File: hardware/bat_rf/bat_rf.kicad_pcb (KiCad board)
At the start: 2 copper layers, 89.8 x 41.5 mm, 95 parts, among them J1 USB_C_Receptacle_PowerOnly_6P, J2 Conn_01x04, J4 Conn_01x02, Q1 NMOS, SW2 RESET, U1 TPS54331, U2 IP2325_5M_WHJC, U3 ESP8684-WROOM-02UC

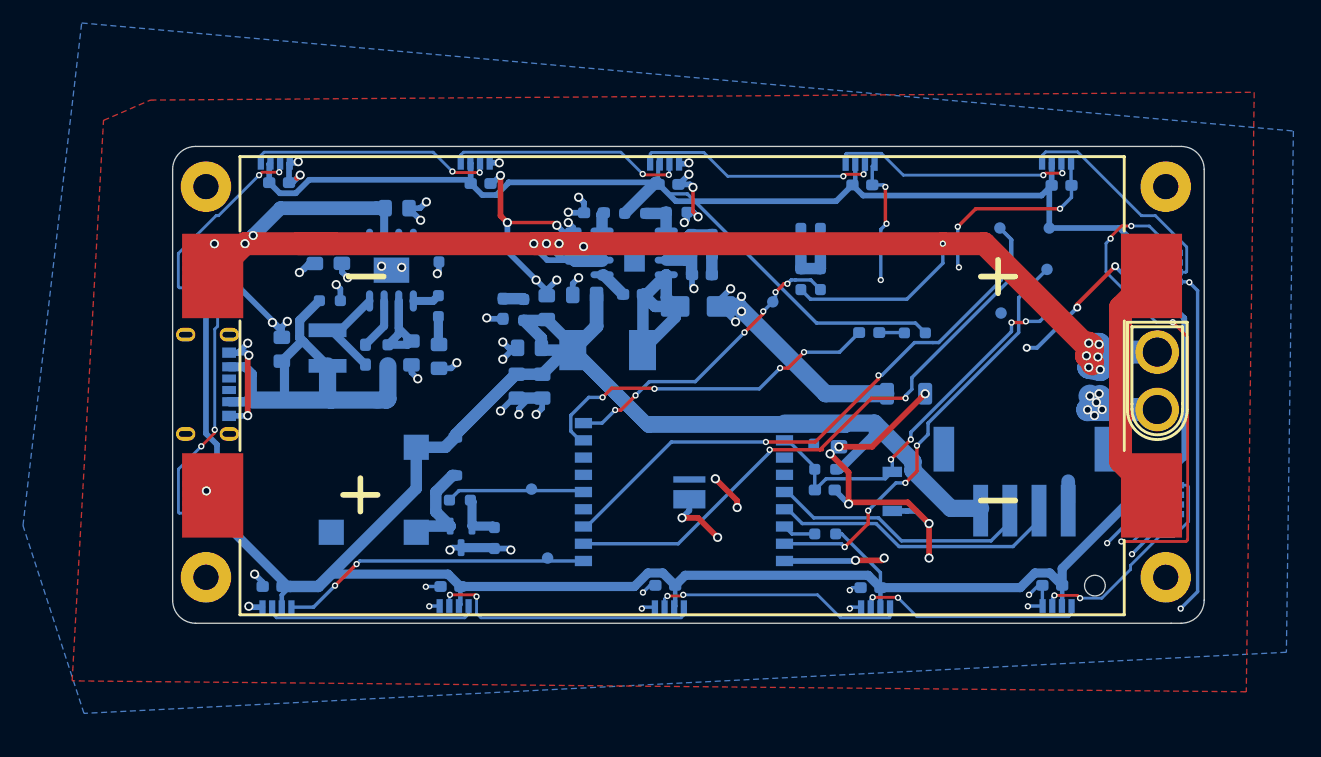
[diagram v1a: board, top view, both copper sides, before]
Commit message: update rfBat
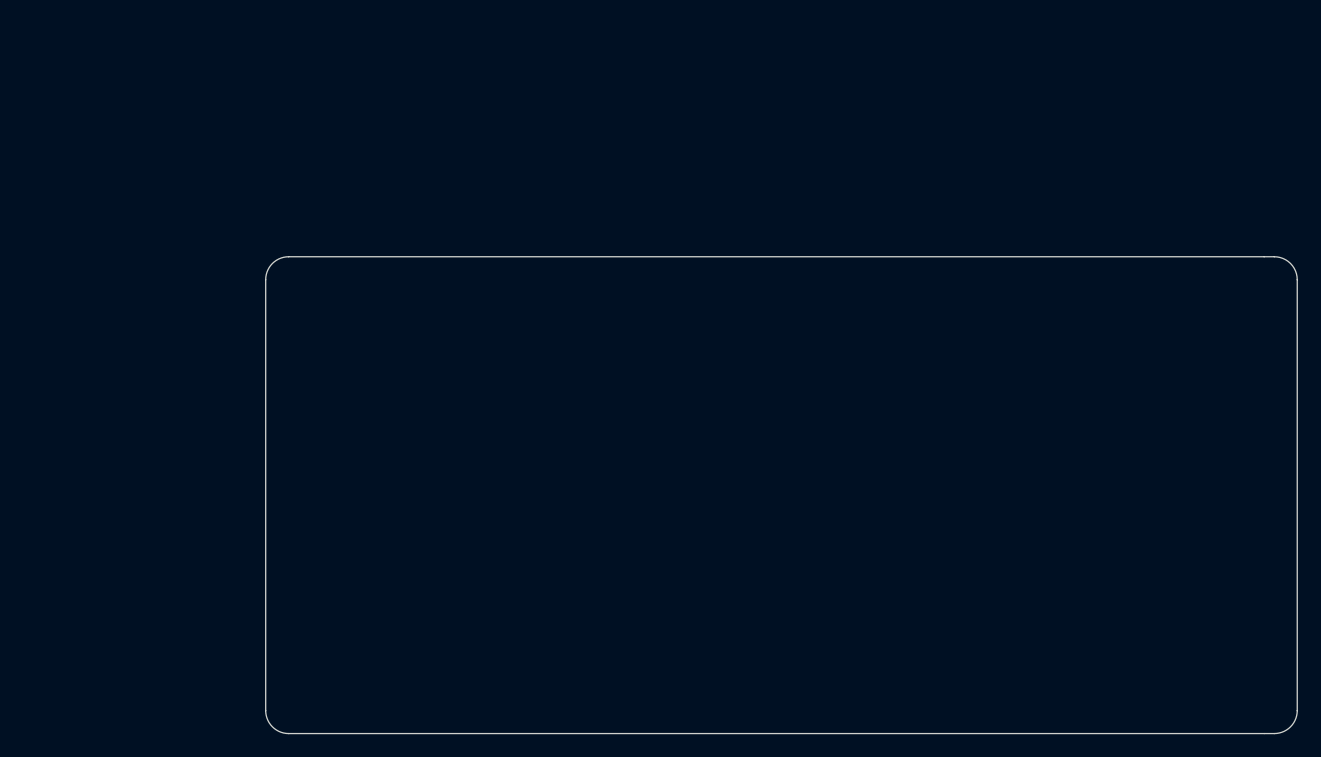
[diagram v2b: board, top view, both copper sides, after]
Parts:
- removed BT2: doubleBatCell, bat_rf:BAT-SMD_BH-18650-B1BA007
- removed BZ1: Buzzer, Buzzer_Beeper:MagneticBuzzer_Kobitone_254-EMB84Q-RO
- removed C1, C10, C16, C2, C26, C3, C39, C4: 22u, Capacitor_SMD:C_0805_2012Metric_Pad1.18x1.45mm_HandSolder
- removed C14, C15, C17, C21, C22, C23, C24, C25, C27, C30, C31, C32, C33, C34, C35, C36, C5, C6: 100n, Capacitor_SMD:C_0603_1608Metric_Pad1.08x0.95mm_HandSolder
- removed C18: 8.2n, Capacitor_SMD:C_0603_1608Metric_Pad1.08x0.95mm_HandSolder
- removed C19: 1n, Capacitor_SMD:C_0603_1608Metric_Pad1.08x0.95mm_HandSolder
- removed C20, C28, C29, C40: 10u, Capacitor_SMD:C_0805_2012Metric_Pad1.18x1.45mm_HandSolder
- removed C37: 2.2u, Capacitor_SMD:C_0603_1608Metric_Pad1.08x0.95mm_HandSolder
- removed C38: 10p, Capacitor_SMD:C_0603_1608Metric_Pad1.08x0.95mm_HandSolder
- removed D12: 3A, Diode_SMD:D_SMA
- removed D13, D14: LED, LED_SMD:LED_0603_1608Metric_Pad1.05x0.95mm_HandSolder
- removed D2: RED, Capacitor_SMD:C_0805_2012Metric_Pad1.18x1.45mm_HandSolder
- removed D5: 1N4148W, Diode_SMD:D_SOD-123
- removed FB1: FerriteBead, Inductor_SMD:L_1206_3216Metric_Pad1.22x1.90mm_HandSolder
- removed H1, H2, H3, H4: MountingHole, MountingHole:MountingHole_2.2mm_M2_Pad
- removed J1: USB_C_Receptacle_PowerOnly_6P, bat_rf:USB-C-SMD_HX-TYPE-C-6PIN
- removed J2: Conn_01x04, bat_rf:CONN-SMD_4P-P2.54_XH2.54-4AB_vertical
- removed J4: Conn_01x02, bat_rf:CONN-TH_XT30U-M
- removed L2: 2.2uH, Inductor_SMD_Wurth:L_Wurth_WE-LQSH-4020
- removed L3: 4.5u, bat_rf:IND-SMD_L7.0-W6.6_0630CDMCCDS
- removed LED1, LED10, LED11, LED12, LED13, LED14, LED2, LED3, LED4, LED5, LED6, LED7, LED8, LED9: XL-4020RGBC-WS2812B, bat_rf:LED-SMD_4P-L4.0-W1.7_M4020-03003-RGB-862-001
- removed Q1: NMOS, Package_TO_SOT_SMD:SOT-23
- removed R1: 0.5R, Resistor_SMD:R_0603_1608Metric_Pad0.98x0.95mm_HandSolder
- removed R10: 3m, Resistor_SMD:R_0603_1608Metric_Pad0.98x0.95mm_HandSolder
- removed R13, R14, R17: 1k, Resistor_SMD:R_0603_1608Metric_Pad0.98x0.95mm_HandSolder
- removed R15: 10.2k, Resistor_SMD:R_0603_1608Metric_Pad0.98x0.95mm_HandSolder
- removed R16: 3.24k, Resistor_SMD:R_0603_1608Metric_Pad0.98x0.95mm_HandSolder
- removed R18: 51k, Resistor_SMD:R_0603_1608Metric_Pad0.98x0.95mm_HandSolder
- removed R2: 5k1, Resistor_SMD:R_0603_1608Metric_Pad0.98x0.95mm_HandSolder
- removed R3, R6: 100R, Resistor_SMD:R_0603_1608Metric_Pad0.98x0.95mm_HandSolder
- removed R4, R5, R7: 10k, Resistor_SMD:R_0603_1608Metric_Pad0.98x0.95mm_HandSolder
- removed R8: 29.4k, Resistor_SMD:R_0603_1608Metric_Pad0.98x0.95mm_HandSolder
- removed R9: 7m, Resistor_SMD:R_0603_1608Metric_Pad0.98x0.95mm_HandSolder
- removed SW2: RESET, Button_Switch_SMD:SW_SPST_B3U-1000P
- removed TP1, TP2, TP3, TP4, TP5, TP6, TP7, TP8, TP9: TestPoint, TestPoint:TestPoint_Pad_D1.0mm
- removed U1: TPS54331, bat_rf:SOP8-PAD
- removed U2: IP2325_5M_WHJC, bat_rf:ESOP-8_L4.9-W3.9-P1.27-LS6.0-BL-EP3.1
- removed U3: ESP8684-WROOM-02UC, bat_rf:WIFIM-SMD_19P-L18.0-W14.3-P1.50_ESP8684-WROOM-02UC
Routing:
- net +3V3: track 433.4 -> 0.00 mm
- net GNDPWR: track 250.7 -> 0.00 mm, vias 76 -> 0
- net +BATT: track 155.5 -> 0.00 mm, vias 13 -> 0
- net /RXD: track 60.0 -> 0.00 mm, vias 2 -> 0
- net Net-(C28-Pad1): track 53.3 -> 0.00 mm
- net GNDD: track 51.9 -> 0.00 mm, vias 12 -> 0
- net Net-(LED1-DI): track 49.9 -> 0.00 mm, vias 4 -> 0
- net /TXD: track 46.5 -> 0.00 mm, vias 2 -> 0
- net /IO9: track 37.3 -> 0.00 mm, vias 4 -> 0
- net /EN: track 33.8 -> 0.00 mm, vias 4 -> 0
- net /LED: track 30.9 -> 0.00 mm, vias 4 -> 0
- net /RGB: track 27.1 -> 0.00 mm, vias 2 -> 0
- net /ESP_RX: track 27.0 -> 0.00 mm
- net /BAT_FB: track 26.6 -> 0.00 mm, vias 6 -> 0
- net Net-(LED13-DO): track 25.7 -> 0.00 mm, vias 2 -> 0
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- removed copper zone on B.Cu, net GNDD
- removed copper zone on F.Cu, net GNDPWR
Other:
- board text removed: "+3V3"
- board text removed: "+BAT"
- board text removed: "0.0000 mm / 0.0000 mm"
- board text removed: "0.3000 mm"
- board text removed: "1.6000 mm"
- board text removed: "2"
- board text removed: "3V3"
- board text removed: "88.9000 mm x 41.5000 mm"
- board text removed: "BAT_V"
- board text removed: "BEEPER"
- board text removed: "BOARD CHARACTERISTICS"
- board text removed: "BOOT"
- board text removed: "CHARGER"
- board text removed: "DC-DC(3.3V)"
- board text removed: "EN"
- board text removed: "GND"
- board text removed: "LED"
- board text removed: "M2"
- board text removed: "MCU"
- board text removed: "None"
- board text removed: "RESET"
- board text removed: "RGB"
- board text removed: "RX"
- board text removed: "RXD"
- board text removed: "TX"
- board text removed: "TXD"
- board text removed: "V1.2"
- board text removed: "否"
- board text removed: "孔最小直径："
- board text removed: "最小布线/间距："
- board text removed: "板子整体尺寸："
- board text removed: "电路板厚度："
- board text removed: "电镀板边："
- board text removed: "边缘卡连接器："
- board text removed: "邮票孔："
- board text removed: "铜层数量："
- board text removed: "铜表面处理（镀铜）："
- board text removed: "阻抗控制"
